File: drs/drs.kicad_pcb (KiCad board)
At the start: 2 copper layers, 68.5 x 53.5 mm, 21 parts, among them J1 POWER, J2 BUTTON, J3 CAN, J4 SERVO, U1 SN65HVD230, U2 TXU0202

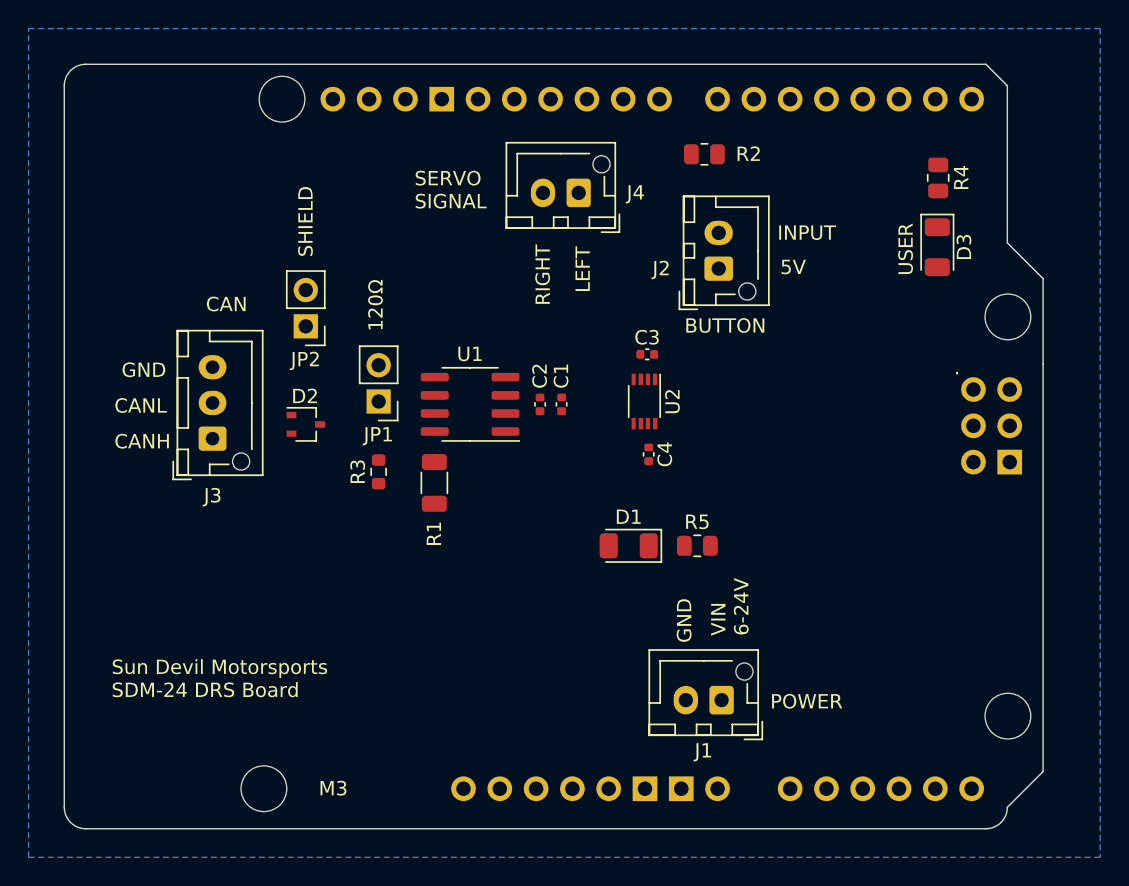
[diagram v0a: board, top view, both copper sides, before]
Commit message: start routing on logger
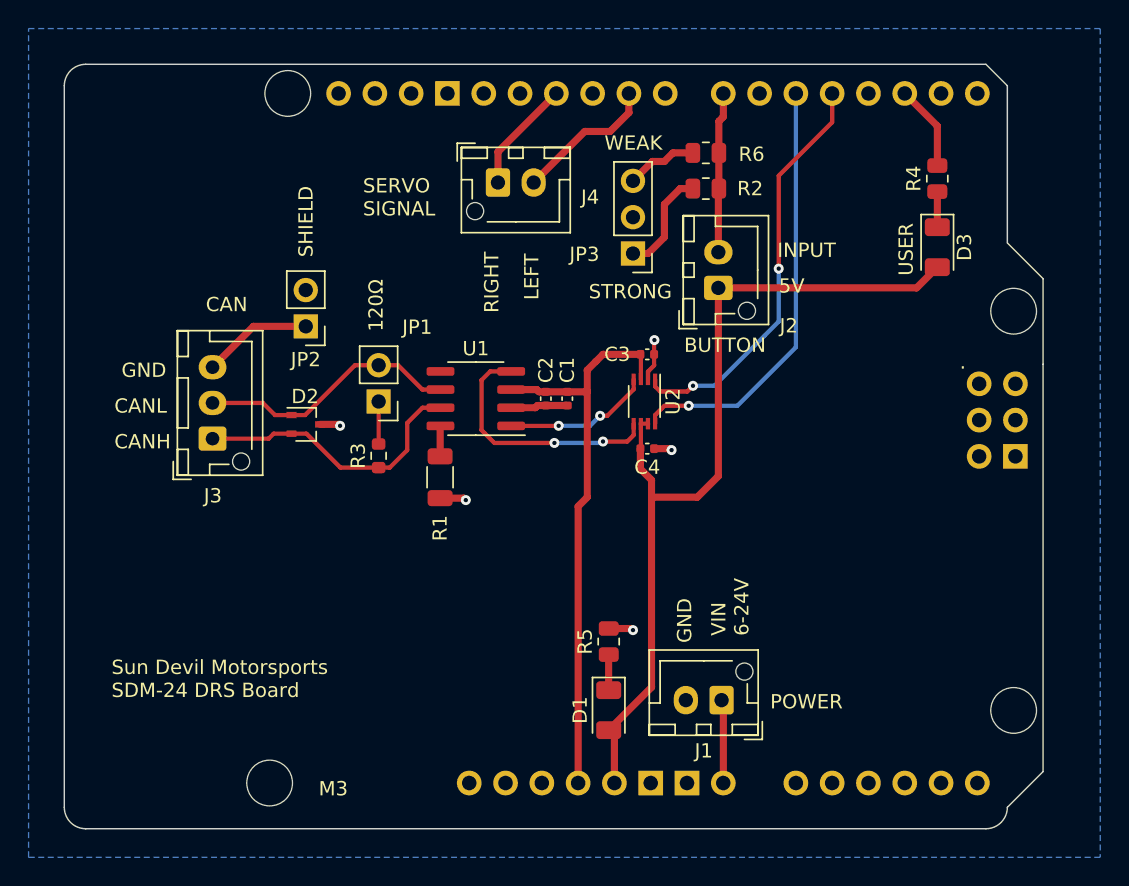
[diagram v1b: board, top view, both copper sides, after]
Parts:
- added JP3: PULLDOWN, Connector_PinHeader_2.54mm:PinHeader_1x03_P2.54mm_Vertical, F.Cu at (154.3, 82.7)
- added R6: 10k, Resistor_SMD:R_0805_2012Metric, F.Cu at (159.4, 75.7)
- moved D1 11.6 mm to (152.6, 114.7), turned to -90 degrees
- moved R5 9.13 mm to (152.6, 109.9), turned to 90 degrees
- moved J4 5.70 mm to (144.8, 77.8), turned to 0 degrees
- moved R2 2.40 mm to (159.4, 78.2)
- moved J2 1.35 mm to (160.3, 85.2)
- moved R3 1.12 mm to (136.5, 96.9)
- moved A1 0.57 mm to (114.9, 122.3)
- moved R1 0.57 mm to (140.8, 98.4)
- moved U1 0.57 mm to (143.3, 92.9)
- moved C1 0.57 mm to (149.7, 92.9)
- moved C2 0.57 mm to (148.2, 92.9)
- moved C4 0.41 mm to (155.3, 96.4), turned to 0 degrees
- moved R4 0.08 mm to (175.6, 77.5), turned to 90 degrees
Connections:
- J4 pad 1: /SERVO_LEFT -> /SERVO_RIGHT
- J4 pad 2: /SERVO_RIGHT -> /SERVO_LEFT
- R2 pad 2: GND -> /STRONG_PULLDOWN
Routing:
- net +5V: track 0.00 -> 61.8 mm
- net +3.3V: track 0.00 -> 40.5 mm
- net /CRX_5V: track 0.00 -> 30.2 mm, vias 0 -> 1
- net /CTX_5V: track 0.00 -> 28.8 mm, vias 0 -> 2
- net /CANH: track 0.00 -> 19.9 mm
- net /CANL: track 0.00 -> 18.5 mm
- net /CRX_3V3: track 0.00 -> 17.9 mm, vias 0 -> 2
- net GND: track 0.00 -> 13.2 mm, vias 0 -> 5
- net /BTN_INPUT: track 0.00 -> 11.3 mm
- net /CTX_3V3: track 0.00 -> 10.3 mm, vias 0 -> 2
- net /SERVO_LEFT: track 0.00 -> 10.0 mm
- net /SERVO_RIGHT: track 0.00 -> 7.93 mm
- net /SHIELD: track 0.00 -> 7.71 mm
- net /STRONG_PULLDOWN: track 0.00 -> 7.42 mm
- net /USR_LED: track 0.00 -> 5.99 mm
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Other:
- board text added: "STRONG"
- board text added: "WEAK"
